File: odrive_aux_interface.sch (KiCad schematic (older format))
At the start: 42 parts, among them J1 Conn_01x20_Male, J10 Conn_01x03, J11 Conn_01x03, J12 Conn_01x06, J13 Conn_01x02, J14 Conn_01x03, J2 Conn_01x03, J3 Conn_01x03, J4 Conn_01x03, J5 Conn_01x03, J6 Conn_01x04, J7 Conn_01x06, J8 Conn_01x03, J9 Conn_01x03, U1 EL814

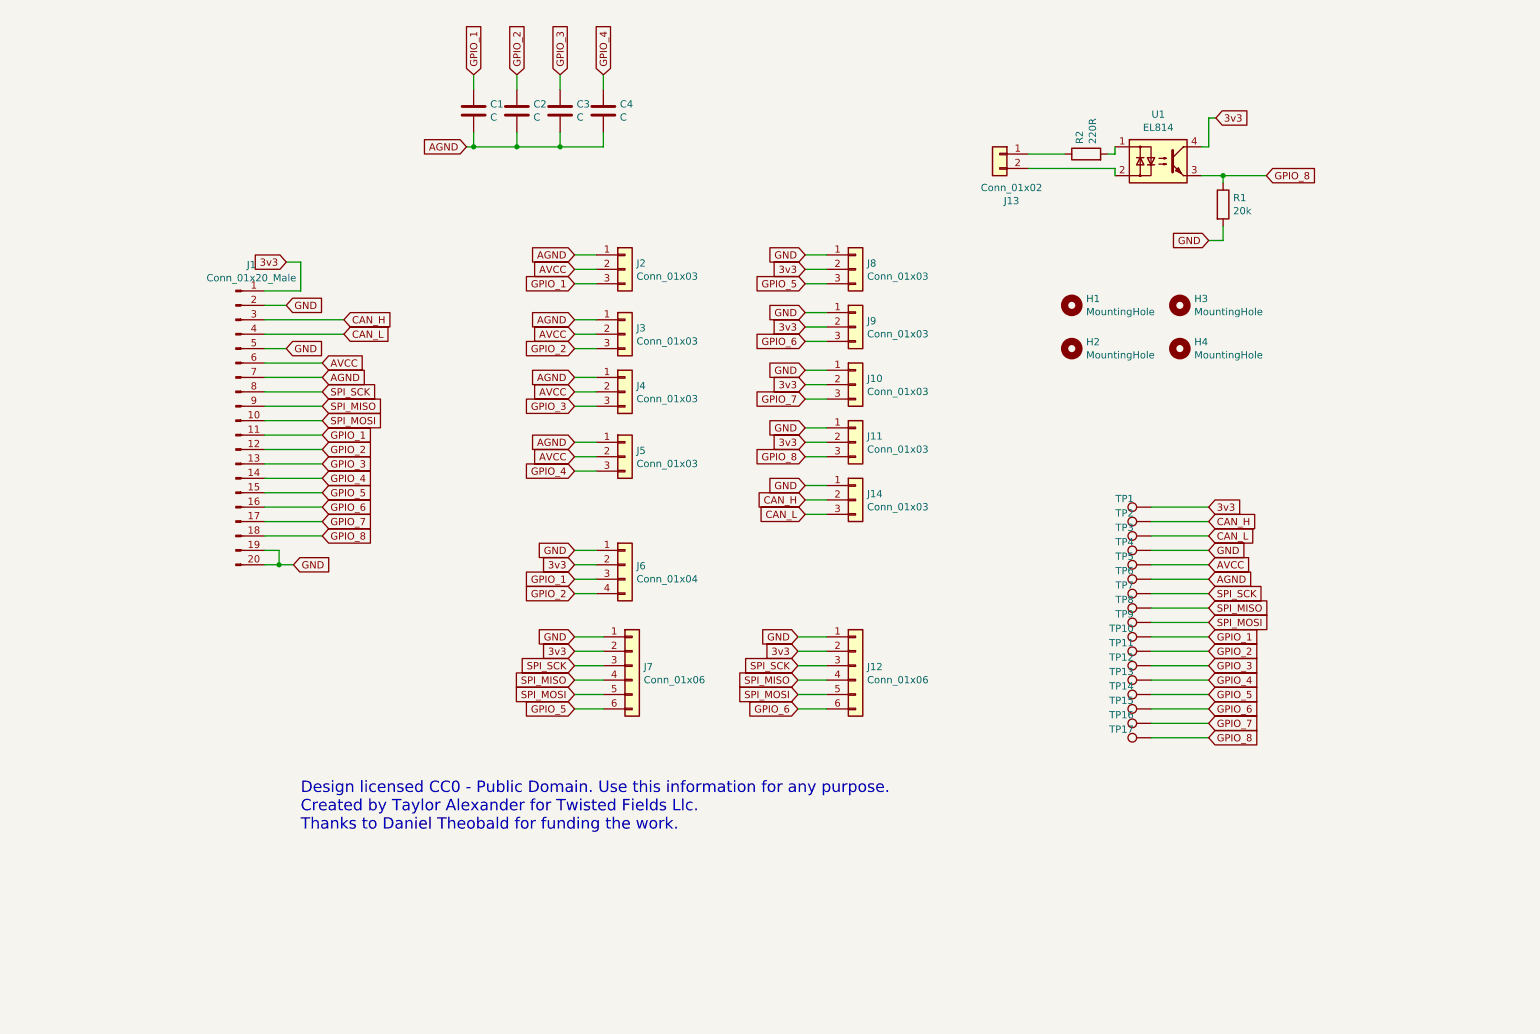
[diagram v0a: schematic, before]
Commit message: Update to v1.2, add gerbers.
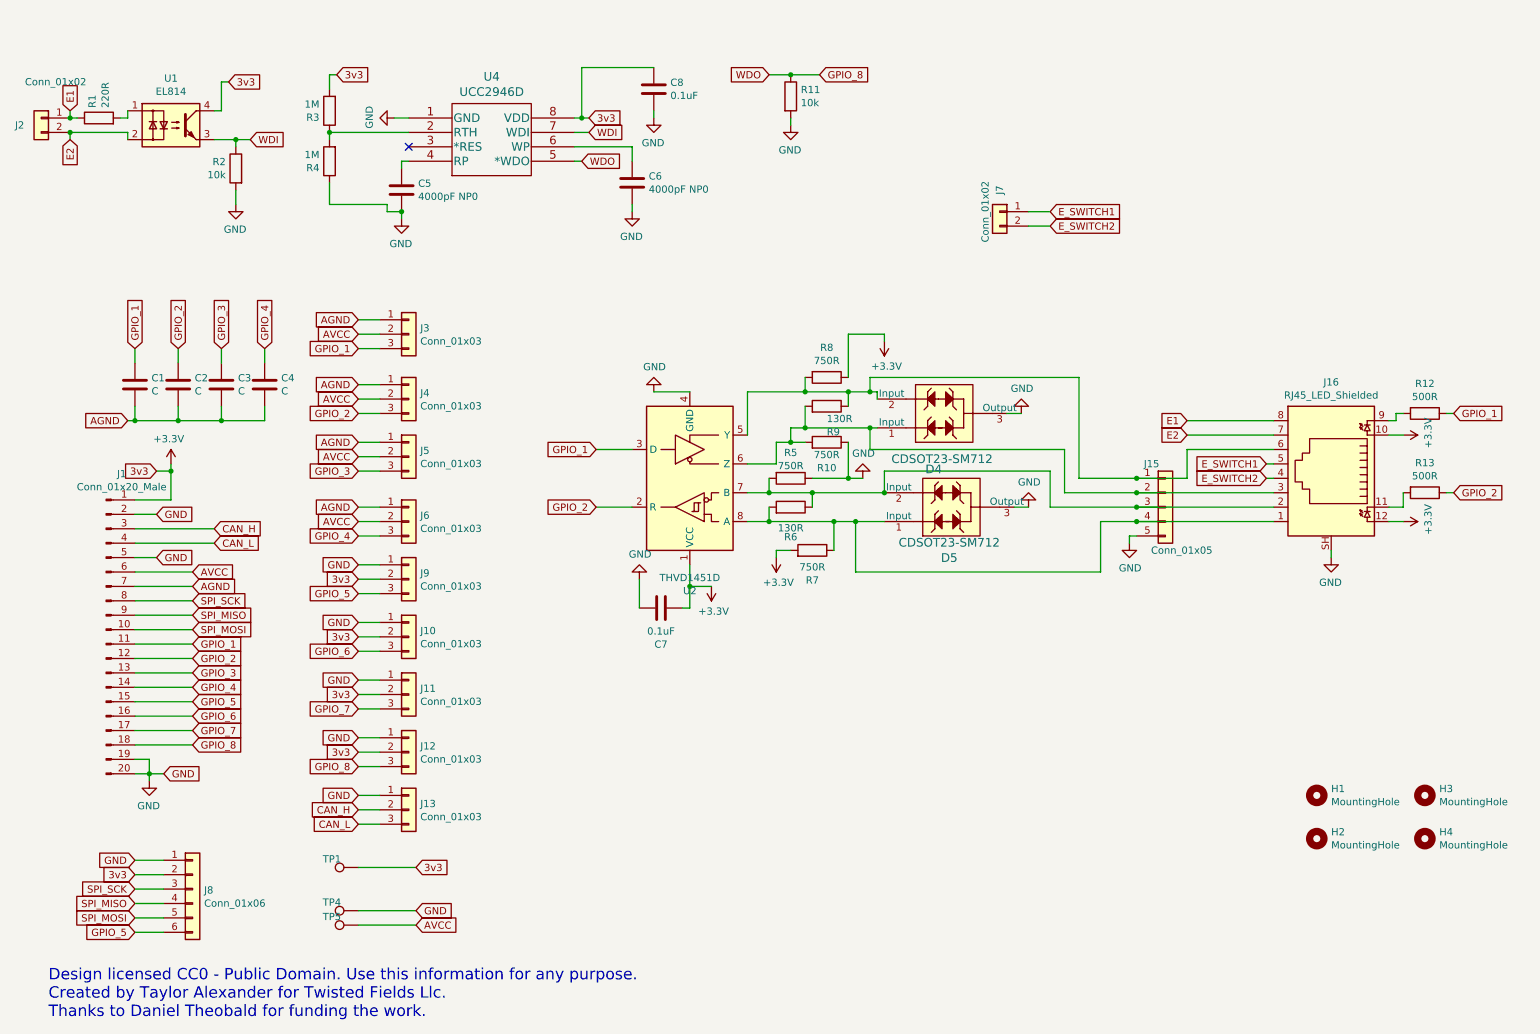
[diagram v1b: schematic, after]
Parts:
- removed J12: Conn_01x06, Connector_JST:JST_XH_B6B-XH-A_1x06_P2.50mm_Vertical, symbol Connector_Generic:Conn_01x06
- removed J6: Conn_01x04, Connector_JST:JST_XH_B4B-XH-A_1x04_P2.50mm_Vertical, symbol Connector_Generic:Conn_01x04
- removed TP10, TP11, TP12, TP13, TP14, TP15, TP16, TP17, TP2, TP3, TP6, TP7, TP8, TP9: TestPoint, TestPoint:TestPoint_Keystone_5015_Micro-Minature, symbol Connector:TestPoint
- added C5, C6: 4000pF NP0, Capacitor_SMD:C_0805_2012Metric, symbol Device:C
- added C7, C8: 0.1uF, Capacitor_SMD:C_0805_2012Metric, symbol Device:C
- added D4, D5: CDSOT23-SM712, digikey-footprints:SOT-23-3, symbol dk_TVS-Diodes:CDSOT23-SM712
- added J15: Conn_01x05, Connector_JST:JST_XH_B5B-XH-A_1x05_P2.50mm_Vertical, symbol Connector_Generic:Conn_01x05
- added J16: RJ45_LED_Shielded, Connector_RJ:RJ45_Amphenol_RJHSE538X, symbol Connector:RJ45_LED_Shielded
- added J7: Conn_01x02, Connector_JST:JST_XH_B2B-XH-A_1x02_P2.50mm_Vertical, symbol Connector_Generic:Conn_01x02
- added R10, R5, R7, R8: 750R, Resistor_SMD:R_0805_2012Metric, symbol Device:R
- added R11: 10k, Resistor_SMD:R_0805_2012Metric, symbol Device:R
- added R12, R13: 500R, Resistor_SMD:R_0805_2012Metric, symbol Device:R
- added R3, R4: 1M, Resistor_SMD:R_0805_2012Metric, symbol Device:R
- added R6, R9: 130R, Resistor_SMD:R_0805_2012Metric, symbol Device:R
- added U2: THVD1451D, Package_SO:SOIC-8_3.9x4.9mm_P1.27mm, symbol Interface_UART:THVD1451D
- added U4: UCC2946D, Package_SO:SO-8_3.9x4.9mm_P1.27mm, symbol 2020-05-28_05-11-16:UCC2946D
- R2: renamed from R1; value 20k -> 10k
- renumbered J9 to J10, J10 to J11, J11 to J12, J14 to J13, J13 to J2, J2 to J3, J3 to J4, J4 to J5, J5 to J6, J7 to J8, J8 to J9, R2 to R1
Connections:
- net GND: now also C5.2, C6.2, C7.2, C8.2, D4.3 (Output), D5.3 (Output), J15.5 (Pin_5), J16.SH, R10.1, R11.2, R4.1, R5.1, U2.4 (GND), U4.1 (GND)
- net GPIO_1: now also R12.1, U2.3 (D)
- net GPIO_2: now also R13.1, U2.2 (R)
- net GPIO_8: now also R11.1, U4.5 (*WDO); no longer R2.1, U1.3
- net E1: now reaches J2.1 (Pin_1), R1.1
- net E1: now also J16.8
- net E2: now reaches J2.2 (Pin_2), U1.2
- net E2: now also J16.7
- net 3v3 renamed +3V3
- net +3V3: now also C7.1, C8.1, J16.10, J16.12, R3.2, R7.2, R8.1, U2.1 (VCC), U4.8 (VDD)
- new net: R3.1, R4.2, U4.2 (RTH)
- new net: C5.1, U4.4 (RP)
- new net: C6.1, U4.6 (WP)
- new net: D4.2 (Input), J15.1 (Pin_1), J16.6, R8.2, R9.1, U2.5 (Y)
- new net: D4.1 (Input), J15.2 (Pin_2), J16.3, R10.2, R9.2, U2.6 (Z)
- new net: D5.2 (Input), J15.3 (Pin_3), J16.2, R5.2, R6.1, U2.7 (B)
- new net: D5.1 (Input), J15.4 (Pin_4), J16.1, R6.2, R7.1, U2.8 (A)
- new net: J16.11, R13.2
- new net: J16.9, R12.2
- new net E_SWITCH1: J16.5, J7.1 (Pin_1)
- new net E_SWITCH2: J16.4, J7.2 (Pin_2)
- new net WDI: R2.1, U1.3, U4.7 (WDI)
- no-connect marks 0 -> 1
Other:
- moved on the sheet: C1, C2, C3, C4, H1, H2, H3, H4, J1, J10, J11, J12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
